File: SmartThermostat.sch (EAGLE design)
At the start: 13 parts

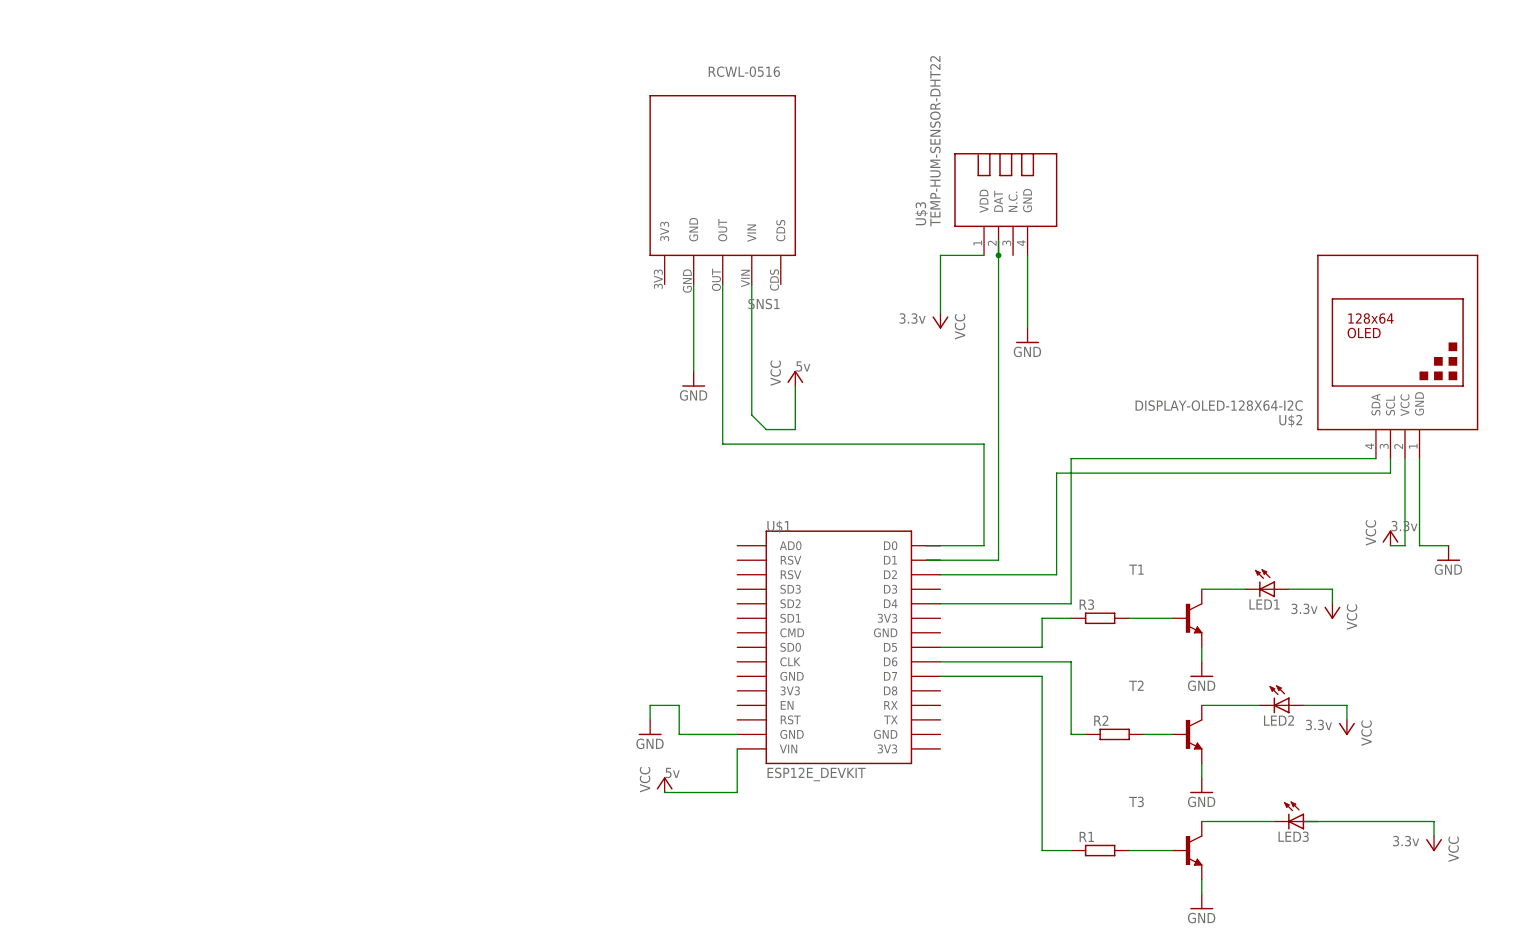
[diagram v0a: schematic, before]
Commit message: updated schematic and readme
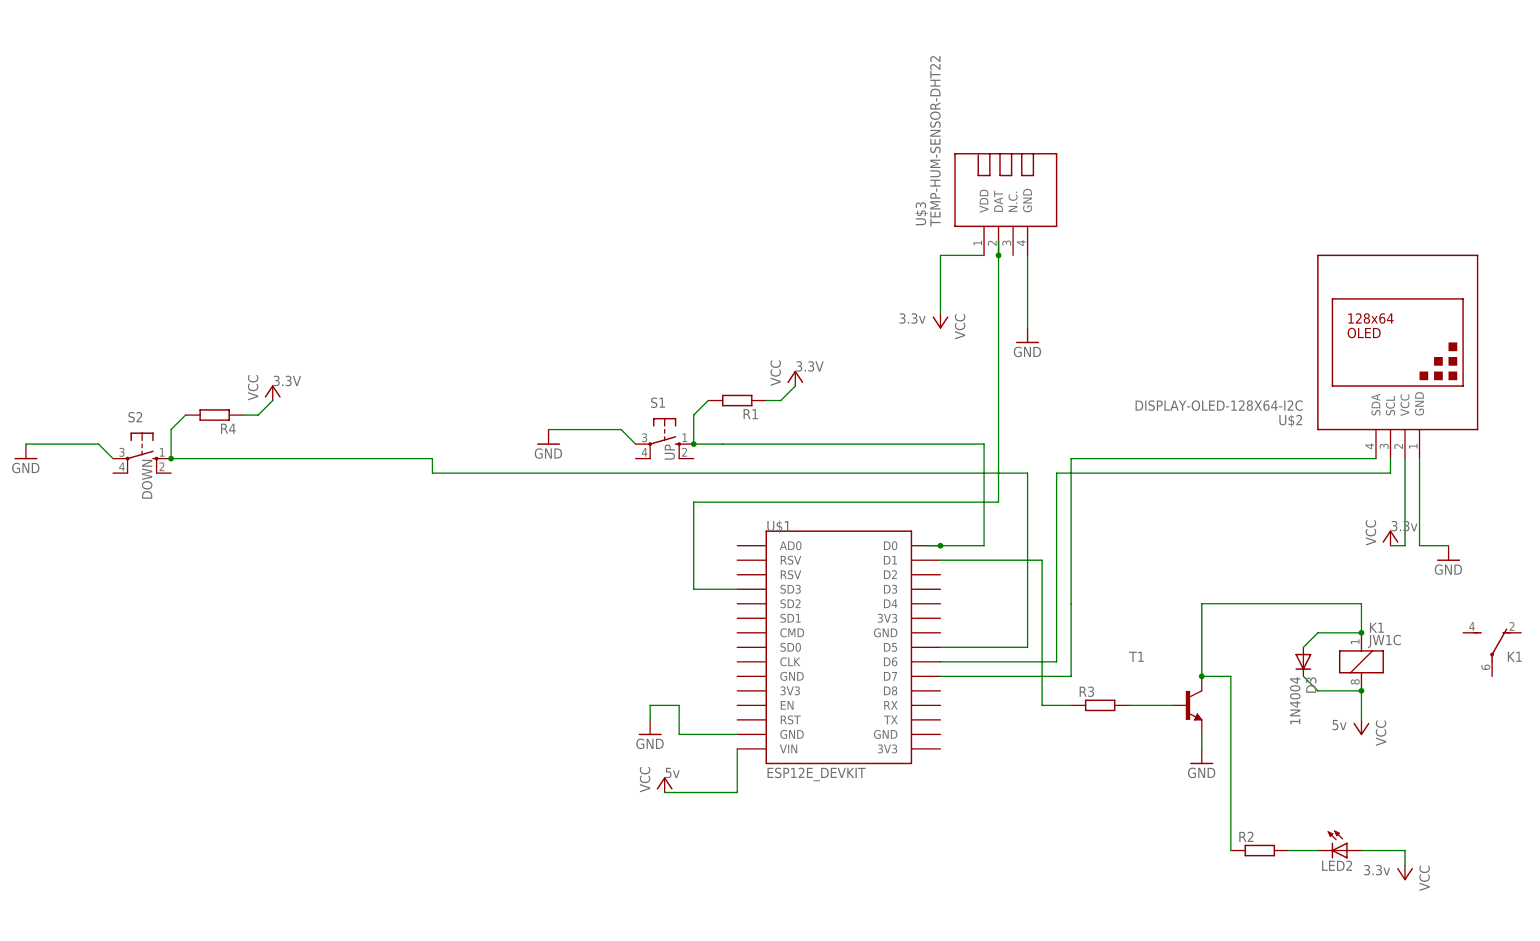
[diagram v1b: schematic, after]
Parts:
- removed LED1, LED3: (no value), eagle-ltspice:LED_ELD260
- removed SNS1: RCWL-0516, RCWL-0516:RCWL-0516
- removed T2, T3: (no value), transistor-neu-to92:2N2222-NPN-TO92-EBC
- added D3: 1N4004, diode:1N4004
- added K1: JW1C, relay:JW1C
- added R4: (no value), eagle-ltspice:R0204/7
- added S1, S2: (no value), switch-omron:10-XX
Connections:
- removed net N$10: LED2.C, T2.C
- removed net N$11: LED1.C, T1.C
- removed net N$12: R3.1, U$1.D5
- removed net N$13: R2.1, U$1.D6
- removed net N$14: R1.1, U$1.D7
- new net N$15: R3.1, U$1.D1
- net GND: now also S1.P, S2.P; no longer SNS1.GND, T2.E, T3.E
- net N$2: now also U$1.D7; no longer U$1.D4
- net N$3: now also U$1.D6; no longer U$1.D2
- net N$4: now also R1.2, S1.S, U$1.D0; no longer SNS1.OUT
- net N$5: now also U$1.SD3
- net N$6: now also LED2.C, R2.2; no longer R1.2, T3.B
- net N$7: now also D3.A, K1_.1, R2.1, T1.C; no longer R2.2, T2.B
- net N$9: now also R4.2, S2.S, U$1.D5; no longer LED3.C, T3.C
- net VCC: now also D3.C, K1_.2, R1.1, R4.1; no longer LED1.A, SNS1.VIN
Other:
- moved on the sheet: LED2, R1, R2, R3, T1
